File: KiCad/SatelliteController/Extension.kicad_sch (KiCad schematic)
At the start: 3 parts, among them J7 CONN_STATUS_PANEL, J8 CONN_PANEL_BAORD_2, J9 CONN_PANEL_BAORD_1

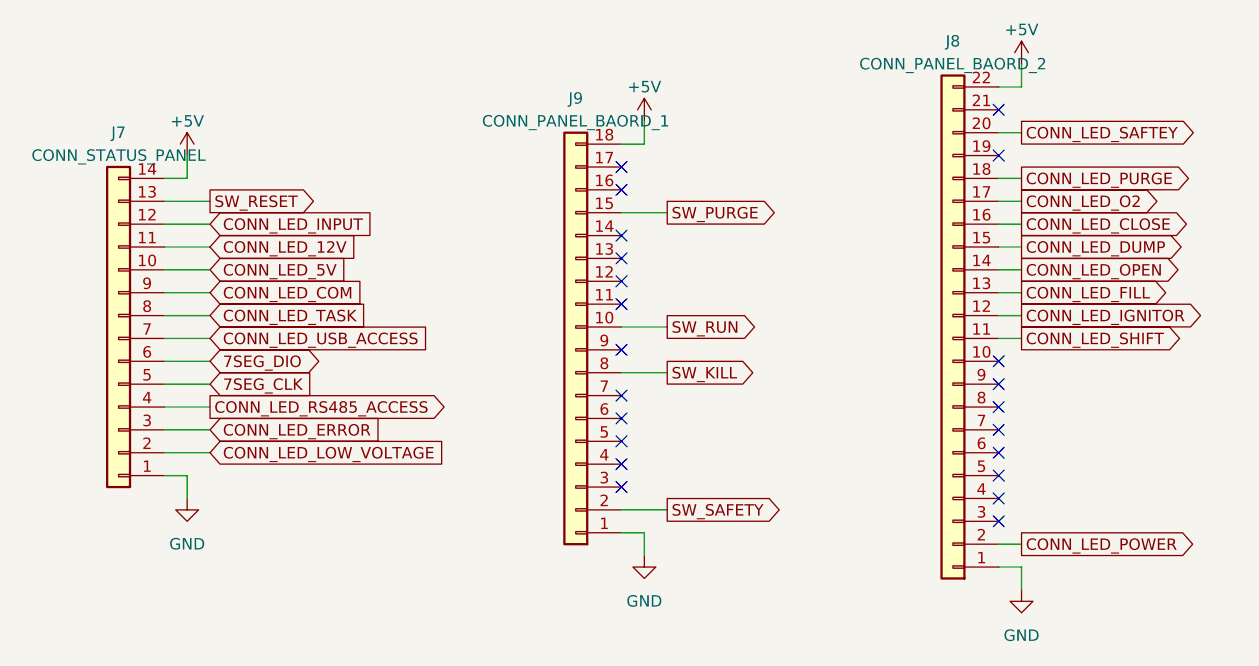
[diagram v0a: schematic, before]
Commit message: コネクタをまとめた
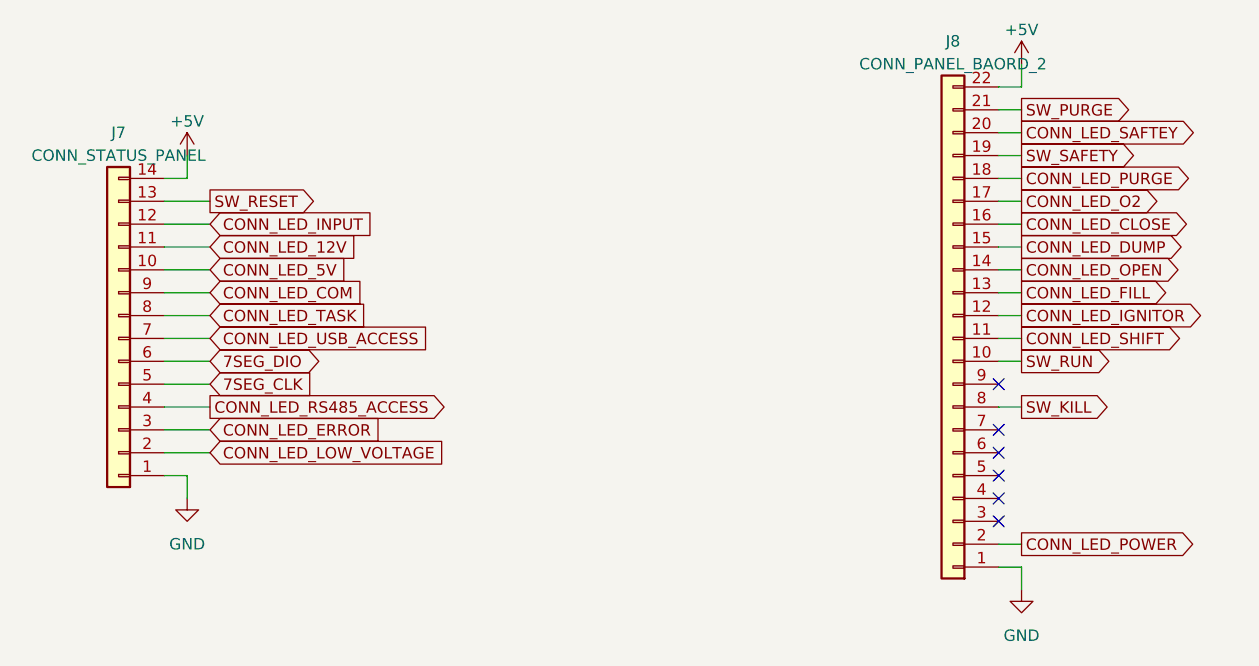
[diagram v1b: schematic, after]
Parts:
- removed J9: CONN_PANEL_BAORD_1, TSRP_Connector_Hirose:DF51A-18DP-2DS, symbol Connector_Generic:Conn_01x18
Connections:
- net SW_KILL: now also J8.8 (Pin_8)
- net SW_PURGE: now also J8.21 (Pin_21)
- net SW_RUN: now also J8.10 (Pin_10)
- net SW_SAFETY: now also J8.19 (Pin_19)
- no-connect marks 22 -> 6
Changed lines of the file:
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@@
 (kicad_sch (version 20230121) (generator eeschema)
   (paper "A4")
-  (no_connect (at 83.82 49.53))
-  (no_connect (at 83.82 52.07))
-  (no_connect (at 83.82 77.47))
   (no_connect (at 125.73 66.04))
-  (no_connect (at 125.73 40.64))
-  (no_connect (at 83.82 74.93))
-  (no_connect (at 83.82 54.61))
-  (no_connect (at 83.82 67.31))
-  (no_connect (at 125.73 35.56))
-  (no_connect (at 83.82 62.23))
-  (no_connect (at 83.82 44.45))
-  (no_connect (at 125.73 68.58))
   (no_connect (at 125.73 78.74))
-  (no_connect (at 83.82 72.39))
   (no_connect (at 125.73 71.12))
   (no_connect (at 125.73 81.28))
   (no_connect (at 125.73 76.2))
-  (no_connect (at 83.82 69.85))
   (no_connect (at 125.73 73.66))
-  (no_connect (at 125.73 63.5))
-  (no_connect (at 83.82 57.15))
-  (no_connect (at 83.82 41.91))
-  (wire (pts (xy 86.36 36.83) (xy 86.36 39.37))
-    (stroke (width 0) (type default))
-  )
   (wire (pts (xy 125.73 45.72) (xy 128.27 45.72))
     (stroke (width 0) (type default))
@@
     (stroke (width 0) (type default))
   )
+  (wire (pts (xy 125.73 63.5) (xy 128.27 63.5))
+    (stroke (width 0) (type default))
+  )
   (wire (pts (xy 33.02 63.5) (xy 38.1 63.5))
     (stroke (width 0) (type default))
@@
     (stroke (width 0) (type default))
   )
-  (wire (pts (xy 83.82 64.77) (xy 88.9 64.77))
-    (stroke (width 0) (type default))
-  )
   (wire (pts (xy 33.02 53.34) (xy 38.1 53.34))
     (stroke (width 0) (type default))
@@
     (stroke (width 0) (type default))
   )
-  (wire (pts (xy 83.82 80.01) (xy 88.9 80.01))
-    (stroke (width 0) (type default))
-  )
-  (wire (pts (xy 83.82 46.99) (xy 88.9 46.99))
+  (wire (pts (xy 125.73 40.64) (xy 128.27 40.64))
     (stroke (width 0) (type default))
   )
@@
     (stroke (width 0) (type default))
   )
-  (wire (pts (xy 83.82 59.69) (xy 88.9 59.69))
-    (stroke (width 0) (type default))
-  )
   (wire (pts (xy 125.73 83.82) (xy 128.27 83.82))
     (stroke (width 0) (type default))
   )
-  (wire (pts (xy 86.36 39.37) (xy 83.82 39.37))
-    (stroke (width 0) (type default))
-  )
   (wire (pts (xy 35.56 76.2) (xy 35.56 78.74))
     (stroke (width 0) (type default))
   )
-  (wire (pts (xy 86.36 82.55) (xy 86.36 85.09))
-    (stroke (width 0) (type default))
-  )
-  (wire (pts (xy 83.82 82.55) (xy 86.36 82.55))
+  (wire (pts (xy 125.73 68.58) (xy 128.27 68.58))
+    (stroke (width 0) (type default))
+  )
+  (wire (pts (xy 125.73 35.56) (xy 128.27 35.56))
     (stroke (width 0) (type default))
   )
@@
     )
   )
-  (global_label "SW_KILL" (shape output) (at 88.9 64.77 0) (fields_autoplaced)
-    (effects (font (size 1.27 1.27)) (justify left))
-    (property "Intersheetrefs" "${INTERSHEET_REFS}" (at 99.3653 64.77 0)
+  (global_label "SW_KILL" (shape output) (at 128.27 68.58 0) (fields_autoplaced)
+    (effects (font (size 1.27 1.27)) (justify left))
+    (property "Intersheetrefs" "${INTERSHEET_REFS}" (at 138.7353 68.58 0)
       (effects (font (size 1.27 1.27)) (justify left) hide)
     )
@@
     )
   )
-  (global_label "SW_PURGE" (shape output) (at 88.9 46.99 0) (fields_autoplaced)
-    (effects (font (size 1.27 1.27)) (justify left))
-    (property "Intersheetrefs" "${INTERSHEET_REFS}" (at 101.7238 46.99 0)
+  (global_label "SW_PURGE" (shape output) (at 128.27 35.56 0) (fields_autoplaced)
+    (effects (font (size 1.27 1.27)) (justify left))
+    (property "Intersheetrefs" "${INTERSHEET_REFS}" (at 141.0938 35.56 0)
       (effects (font (size 1.27 1.27)) (justify left) hide)
     )
@@
     )
   )
-  (global_label "SW_RUN" (shape output) (at 88.9 59.69 0) (fields_autoplaced)
-    (effects (font (size 1.27 1.27)) (justify left))
-    (property "Intersheetrefs" "${INTERSHEET_REFS}" (at 99.3653 59.69 0)
-      (effects (font (size 1.27 1.27)) (justify left) hide)
-    )
-  )
-  (global_label "SW_SAFETY" (shape output) (at 88.9 80.01 0) (fields_autoplaced)
-    (effects (font (size 1.27 1.27)) (justify left))
-    (property "Intersheetrefs" "${INTERSHEET_REFS}" (at 102.0262 80.01 0)
+  (global_label "SW_RUN" (shape output) (at 128.27 63.5 0) (fields_autoplaced)
+    (effects (font (size 1.27 1.27)) (justify left))
+    (property "Intersheetrefs" "${INTERSHEET_REFS}" (at 138.7353 63.5 0)
+      (effects (font (size 1.27 1.27)) (justify left) hide)
+    )
+  )
+  (global_label "SW_SAFETY" (shape output) (at 128.27 40.64 0) (fields_autoplaced)
+    (effects (font (size 1.27 1.27)) (justify left))
+    (property "Intersheetrefs" "${INTERSHEET_REFS}" (at 141.3962 40.64 0)
       (effects (font (size 1.27 1.27)) (justify left) hide)
     )
@@
     )
   )
-  (symbol (lib_id "Connector_Generic:Conn_01x18") (at 78.74 62.23 180) (unit 1)
-    (in_bom yes) (on_board yes) (dnp no) (fields_autoplaced)
-    (property "Reference" "J9" (at 78.74 34.29 0)
-      (effects (font (size 1.27 1.27)))
-    )
-    (property "Value" "CONN_PANEL_BAORD_1" (at 78.74 36.83 0)
-      (effects (font (size 1.27 1.27)))
-    )
-    (property "Footprint" "TSRP_Connector_Hirose:DF51A-18DP-2DS" (at 78.74 62.23 0)
-      (effects (font (size 1.27 1.27)) hide)
-    )
-    (property "Datasheet" "~" (at 78.74 62.23 0)
-      (effects (font (size 1.27 1.27)) hide)
-    )
-    (property "LCSC" "" (at 78.74 62.23 0)
-      (effects (font (size 1.27 1.27)) hide)
-    )
-    (pin "1")
-    (pin "10")
-    (pin "11")
-    (pin "12")
-    (pin "13")
-    (pin "14")
-    (pin "15")
-    (pin "16")
-    (pin "17")
-    (pin "18")
-    (pin "2")
-    (pin "3")
-    (pin "4")
-    (pin "5")
-    (pin "6")
-    (pin "7")
-    (pin "8")
-    (pin "9")
-    (instances
-      (project "SatelliteController"
-        (path "/628d040b-43bf-4733-804f-091644a90124/7294b7f8-79a7-4ea3-8687-92a673d94882"
-          (reference "J9") (unit 1)
-        )
-      )
-    )
-  )
-  (symbol (lib_id "power:+5V") (at 86.36 36.83 0) (unit 1)
-    (in_bom yes) (on_board yes) (dnp no) (fields_autoplaced)
-    (property "Reference" "#PWR046" (at 86.36 40.64 0)
-      (effects (font (size 1.27 1.27)) hide)
-    )
-    (property "Value" "+5V" (at 86.36 33.02 0)
-      (effects (font (size 1.27 1.27)))
-    )
-    (property "Footprint" "" (at 86.36 36.83 0)
-      (effects (font (size 1.27 1.27)) hide)
-    )
-    (property "Datasheet" "" (at 86.36 36.83 0)
-      (effects (font (size 1.27 1.27)) hide)
-    )
-    (pin "1")
-    (instances
-      (project "SatelliteController"
-        (path "/628d040b-43bf-4733-804f-091644a90124"
-          (reference "#PWR046") (unit 1)
-        )
-        (path "/628d040b-43bf-4733-804f-091644a90124/7294b7f8-79a7-4ea3-8687-92a673d94882"
-          (reference "#PWR049") (unit 1)
-        )
-      )
-    )
-  )
   (symbol (lib_id "power:+5V") (at 128.27 30.48 0) (unit 1)
     (in_bom yes) (on_board yes) (dnp no) (fields_autoplaced)
@@
         )
       )
-    )
-  )
-  (symbol (lib_id "power:GND") (at 86.36 85.09 0) (unit 1)
-    (in_bom yes) (on_board yes) (dnp no) (fields_autoplaced)
-    (property "Reference" "#PWR052" (at 86.36 91.44 0)
-      (effects (font (size 1.27 1.27)) hide)
-    )
-    (property "Value" "GND" (at 86.36 90.17 0)
-      (effects (font (size 1.27 1.27)))
-    )
-    (property "Footprint" "" (at 86.36 85.09 0)
-      (effects (font (size 1.27 1.27)) hide)
-    )
-    (property "Datasheet" "" (at 86.36 85.09 0)
-      (effects (font (size 1.27 1.27)) hide)
-    )
-    (pin "1")
-    (instances
-      (project "SatelliteController"
-        (path "/628d040b-43bf-4733-804f-091644a90124/7294b7f8-79a7-4ea3-8687-92a673d94882"
-          (reference "#PWR052") (unit 1)
-        )
-      )
